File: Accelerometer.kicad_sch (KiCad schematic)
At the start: 2 parts, among them J24 Conn_01x04

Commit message: done ✅
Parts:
- J24: footprint (none) -> Connector_JST:JST_GH_SM04B-GHS-TB_1x04-1MP_P1.25mm_Horizontal
- TP5: footprint TestPoint:TestPoint_Pad_D1.5mm -> TestPoint:TestPoint_Pad_D1.0mm
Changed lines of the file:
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@@
 			)
 		)
-		(property "Footprint" "TestPoint:TestPoint_Pad_D1.5mm"
+		(property "Footprint" "TestPoint:TestPoint_Pad_D1.0mm"
 			(at 154.94 95.25 0)
 			(effects
@@
 			)
 		)
-		(property "Footprint" ""
+		(property "Footprint" "Connector_JST:JST_GH_SM04B-GHS-TB_1x04-1MP_P1.25mm_Horizontal"
 			(at 168.91 95.25 0)
 			(effects

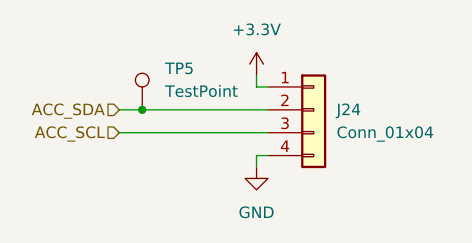
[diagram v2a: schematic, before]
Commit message: First Draft of BOM
Didn't select some compoentns like diodes that I don't fully understand. Also, some components have multiple variants so we must be careful.
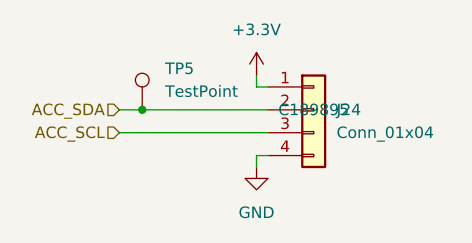
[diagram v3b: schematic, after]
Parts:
- J24: JLC# (none) -> C189895
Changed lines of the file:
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@@
+			)
+		)
+		(property "JLC#" ""
+			(at 149.86 95.25 0)
+			(effects
+				(font
+					(size 1.27 1.27)
+				)
 			)
 		)
@@
 			)
 		)
+		(property "JLC#" "C189895"
+			(at 168.91 95.25 0)
+			(effects
+				(font
+					(size 1.27 1.27)
+				)
+			)
+		)

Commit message: parts⚙️
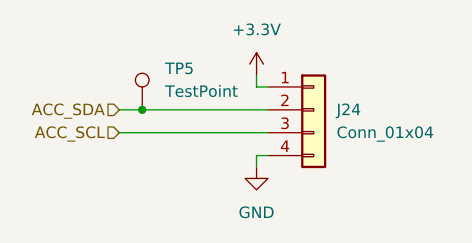
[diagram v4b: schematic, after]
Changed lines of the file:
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@@
 					(size 1.27 1.27)
 				)
+				(hide yes)
 			)
 		)
